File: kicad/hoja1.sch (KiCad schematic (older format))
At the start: 1 part

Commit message: creacion bus y libreria
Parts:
- removed U?: STM32F446ZETx, LQFP144, symbol STM32F446ZETx
- added U?: STM32F446ZETx, Housings_QFP:LQFP-144_20x20mm_Pitch0.5mm, symbol STM32F446ZETx
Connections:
- net labels added: FMC[15:0]
- wire segments 0 -> 16
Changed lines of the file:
@@
 LIBS:stm32
 LIBS:Lattice
+LIBS:stm32f446zetx
 LIBS:design_emb-cache
 EELAYER 25 0
@@
 $Comp
 L STM32F446ZETx U?
-U 1 1 5B7DAF5C
-P 16500 8900
-F 0 "U?" H 12000 12625 50  0000 L BNN
-F 1 "STM32F446ZETx" H 21000 12625 50  0000 R BNN
-F 2 "LQFP144" H 21000 12575 50  0001 R TNN
-F 3 "" H 16500 8900 50  0001 C CNN
-	1    16500 8900
+U 1 1 5B7F8688
+P 23700 16600
+F 0 "U?" H 19200 20325 50  0000 L BNN
+F 1 "STM32F446ZETx" H 28200 20325 50  0000 R BNN
+F 2 "Housings_QFP:LQFP-144_20x20mm_Pitch0.5mm" H 28200 20275 50  0001 R TNN
+F 3 "" H 23700 16600 50  0001 C CNN
+	1    23700 16600
 	1    0    0    -1
 $EndComp
+Wire Bus Line
+	18550 19000 18350 19000
+Text HLabel 18350 19000 0    60   Input ~ 0
+FMC[15:0]
+Entry Bus Bus
+	18550 19800 18650 19900
+Entry Bus Bus
+	18550 19700 18650 19800
+Entry Bus Bus
+	18550 19600 18650 19700
+Entry Bus Bus
+	18550 19500 18650 19600
+Entry Bus Bus
+	18550 19400 18650 19500
+Entry Bus Bus
+	18550 19300 18650 19400
+Entry Bus Bus
+	18550 19200 18650 19300
+Entry Bus Bus
+	18550 19100 18650 19200
+Entry Bus Bus
+	18550 19000 18650 19100
+Wire Bus Line
+	18550 19800 18550 19000
+Wire Bus Line
+	28950 18300 29150 18300
+Wire Wire Line
+	28400 19200 28850 19200
+Wire Wire Line
+	28400 19300 28850 19300
+Wire Wire Line
+	28400 19400 28850 19400
+Text HLabel 29150 18300 2    60   Input ~ 0
+FMC[15:0]
+Entry Bus Bus
+	28950 19800 28850 19900
+Entry Bus Bus
+	28950 19700 28850 19800
+Entry Bus Bus
+	28950 19300 28850 19400
+Entry Bus Bus
+	28950 19200 28850 19300
+Entry Bus Bus
+	28950 19100 28850 19200
+Entry Bus Bus
+	28950 18400 28850 18500
+Entry Bus Bus
+	28950 18300 28850 18400
+Wire Wire Line
+	28400 18400 28850 18400
+Wire Wire Line
+	28400 18500 28850 18500
+Wire Wire Line
+	28400 19800 28850 19800
+Wire Wire Line
+	28400 19900 28850 19900
+Wire Bus Line
+	28950 18300 28950 19800
+Wire Wire Line
+	19000 19900 18650 19900
+Wire Wire Line
+	18650 19800 19000 19800
+Wire Wire Line
+	19000 19700 18650 19700
+Wire Wire Line
+	19000 19600 18650 19600
+Wire Wire Line
+	19000 19500 18650 19500
+Wire Wire Line
+	19000 19400 18650 19400
+Wire Wire Line
+	19000 19300 18650 19300
+Wire Wire Line
+	19000 19200 18650 19200
+Wire Wire Line
+	19000 19100 18650 19100
 $EndSCHEMATC

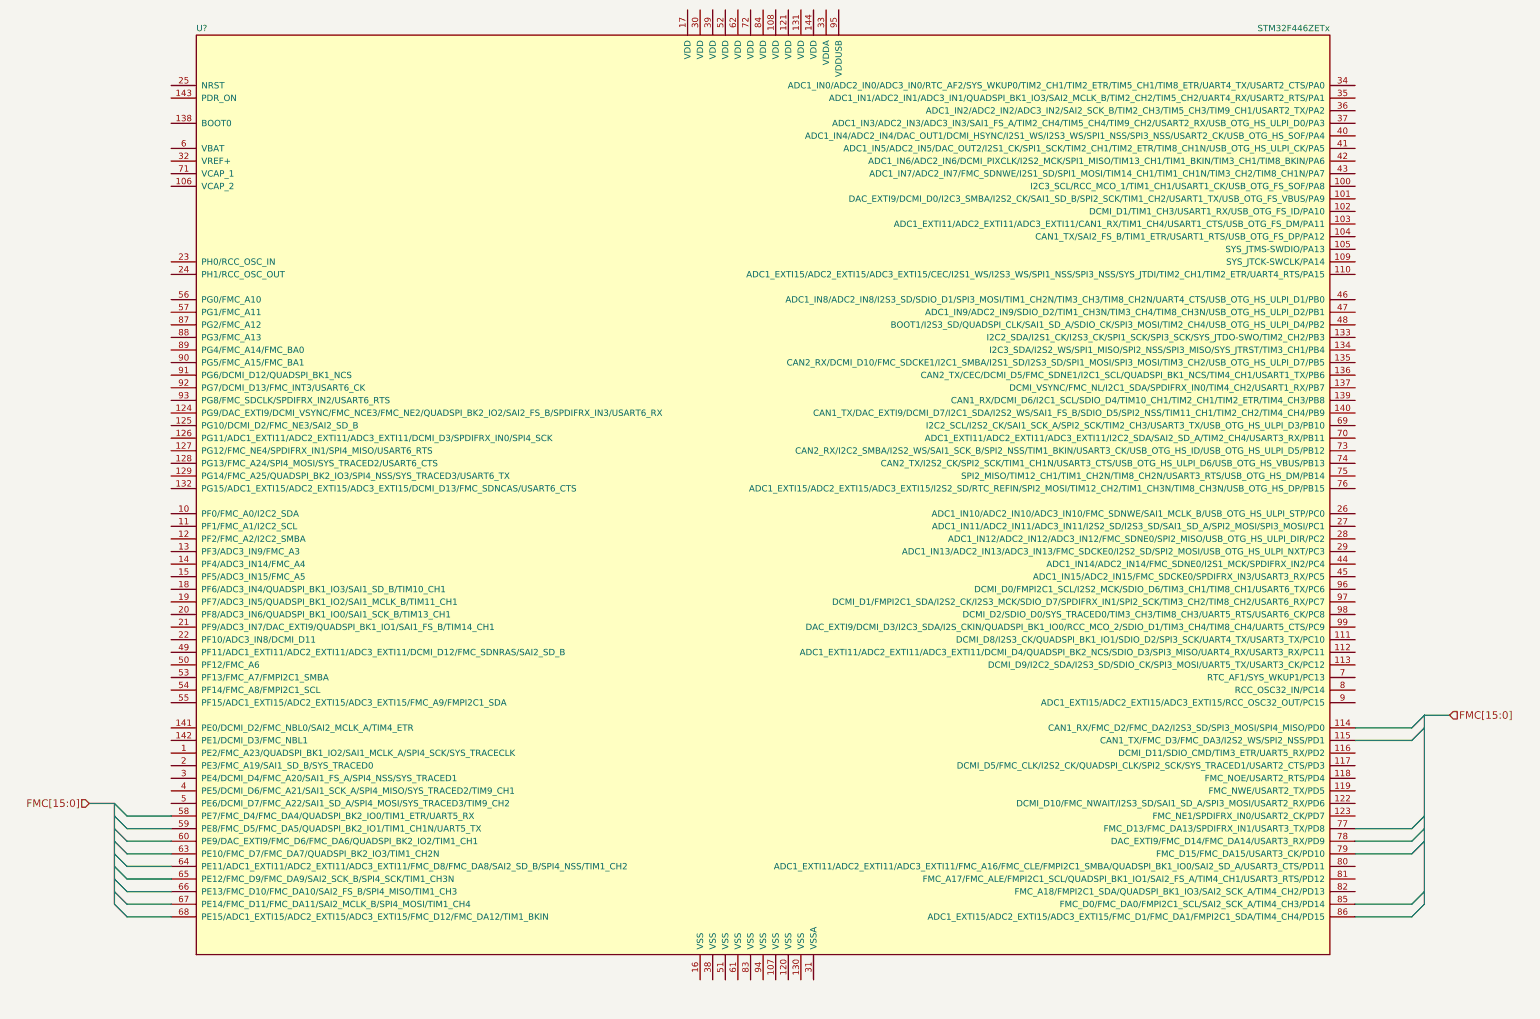
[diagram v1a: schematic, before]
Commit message: creacion bus FMC
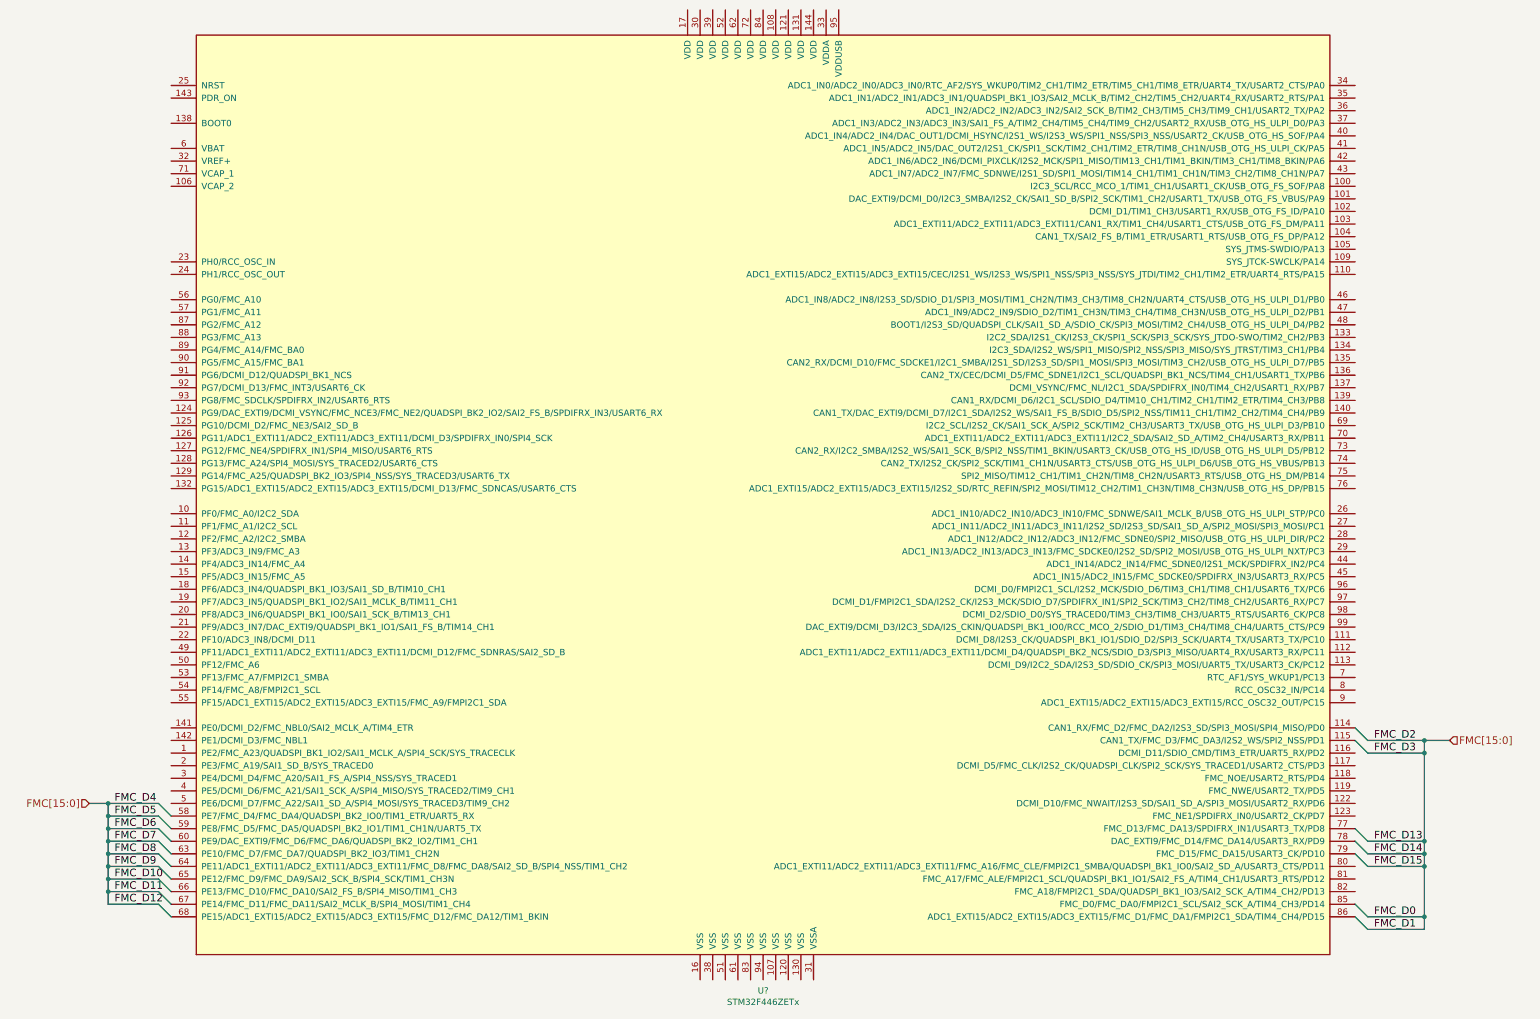
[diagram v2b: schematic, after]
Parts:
- removed U?: STM32F446ZETx, Housings_QFP:LQFP-144_20x20mm_Pitch0.5mm, symbol STM32F446ZETx
- added U?: STM32F446ZETx, Package_QFP:LQFP-144_20x20mm_P0.5mm, symbol stm32:STM32F446ZETx
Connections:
- net labels added: FMC_D0, FMC_D1, FMC_D10, FMC_D11, FMC_D12, FMC_D13, FMC_D14, FMC_D15, FMC_D2, FMC_D3, FMC_D4, FMC_D5, FMC_D6, FMC_D7, FMC_D8, FMC_D9
- wire segments 16 -> 0
